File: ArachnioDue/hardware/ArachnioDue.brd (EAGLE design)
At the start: 17.8 x 58.4 mm, 70 parts, among them J5 HEAD17-NOSS, J6 HEAD17-NOSS, Q1 12MHz, U1 SAM3SA-MU, U2 AP2111HA-3.3, U5 ESP8266EX, U6 SPI_FLASH, Y1 26 MHz/10 pF

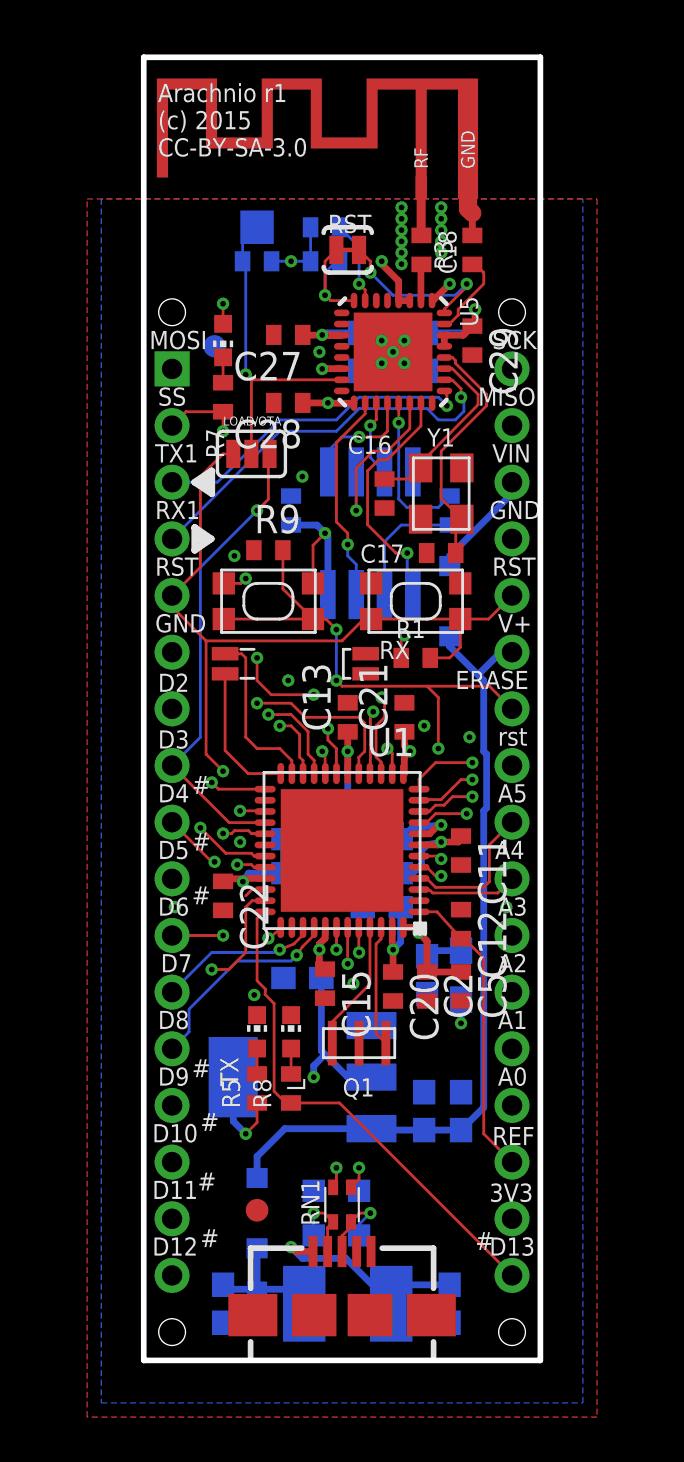
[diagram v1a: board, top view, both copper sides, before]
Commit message: first module version, ready for mfg
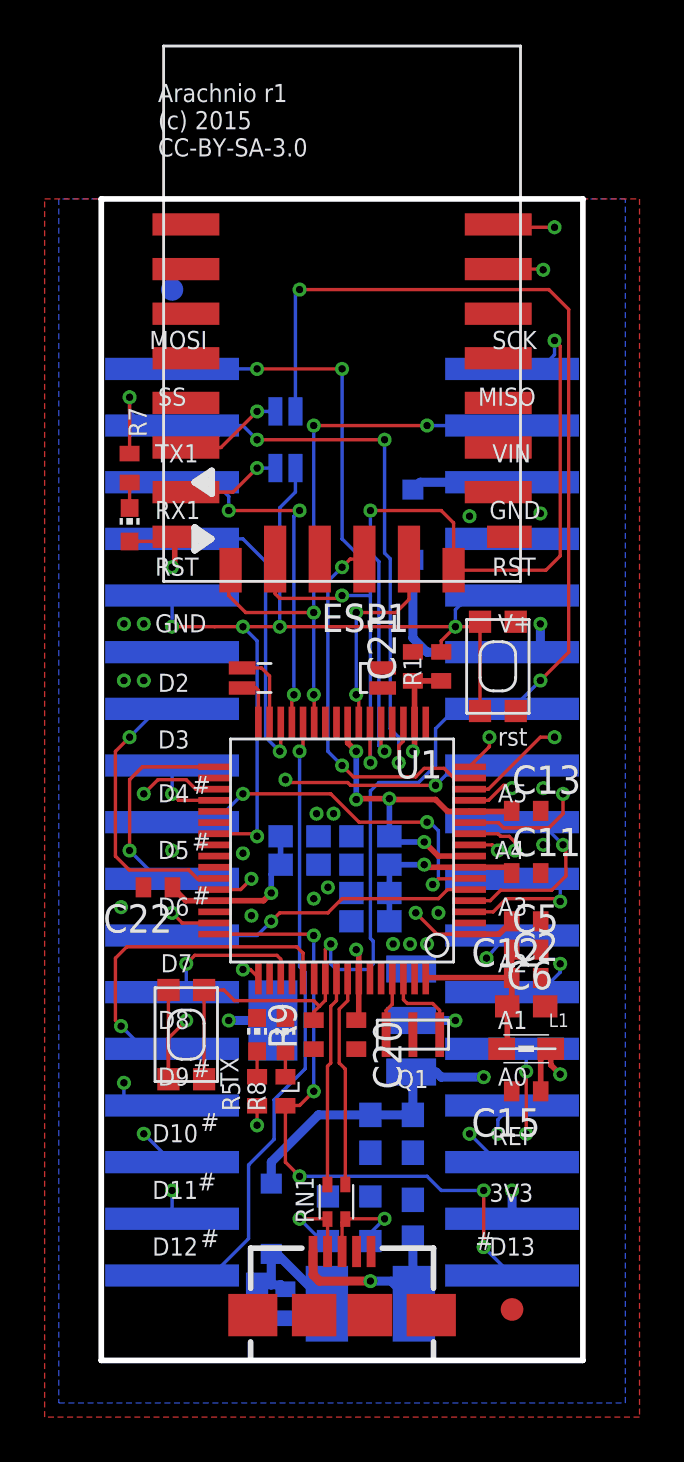
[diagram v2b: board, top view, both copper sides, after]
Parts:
- removed C16, C17: 10 pF, resistor:C0402
- removed C18: 5p6, resistor:C0402
- removed C19, C27, C28, C29: 100n, resistor:C0402
- removed C25, C26: 4u7, resistor:C0603
- removed LOAD/OTA: (no value), SparkFun-Passives:PAD-JUMPER-3-NO_YES_SILK
- removed R10, R11, R14: 10K, resistor:R0402
- removed R13: 200R, resistor:R0402
- removed R3: 12K, resistor:R0402
- removed RST: (no value), SparkFun-Passives:PAD-JUMPER-2-NC_BY_TRACE_YES_SILK
- removed TP3: PTR1TP15SQ, testpad:TP15SQ
- removed U$11: ANTENNA_1RIGHT, ant-planar-1:SWRA117D_RIGHT
- removed U5: ESP8266EX, ESP8266:QFN32
- removed U6: SPI_FLASH, ESP8266:SOIC-8
- removed Y1: 26 MHz/10 pF, SmartPrj:CRYSTAL-3.2-2.5
- added ERASE_JMP, RST_JMP: JUMPER-PAD-2-NOYES_SILK, SparkFun-Passives:PAD-JUMPER-2-NO_YES_SILK
- added ESP1: ESP-12, esp8266-parts:ESP-12
- J5: value HEAD17-NOSS -> (none); device SmartPrj:HEAD17-NOSS -> logos-headers:1X17SMD-UNIVERSAL
- J6: device SmartPrj:HEAD17-NOSS-1 -> logos-headers:1X17SMD-UNIVERSAL
- U1: value SAM3SA-MU -> SAM3SB-AU; device atmel-sam3s:QFN48 -> atmel-sam3s:LQFP64
- moved R9 21.8 mm to (7.62, 14.6), turned to 90 degrees
- moved ERASE 19.8 mm to (1.91, 14.6), turned to 90 degrees
- moved U$12 15.1 mm to (17.1, 48.3)
- moved U$37 12.3 mm to (16.5, 2.29)
- moved C15 10.2 mm to (17.1, 12.1), turned to 180 degrees
- moved RX 9.26 mm to (-0.64, 37.5), turned to 0 degrees
- moved C13 9.03 mm to (17.1, 24.6), turned to 0 degrees
- moved U$1 6.25 mm to (14.6, 41.3)
- moved R7 5.26 mm to (-0.64, 40.0), turned to 270 degrees
- moved RESET 4.70 mm to (15.9, 31.1), turned to 270 degrees
- moved C6 4.66 mm to (17.1, 15.9), flipped to the top, turned to 0 degrees
- moved C2 4.46 mm to (17.1, 17.1), turned to 0 degrees
- moved L1 4.41 mm to (17.1, 14.0), flipped to the top, turned to 180 degrees
- moved C8 4.15 mm to (12.1, 6.35), turned to 90 degrees
- moved C1 3.97 mm to (10.2, 19.7)
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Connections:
- removed net DVDD: U5.24
- removed net N$27: C17.1, U5.28, Y1.1
- removed net N$28: C16.1, U5.27, Y1.3
- removed net N$31: C18.1, U$11.RF
- removed net N$32: R3.1, U5.31
- removed net N$33: RST.1, U5.32
- removed net N$34: R13.2, U5.21
- removed net N$35: R13.1, U6.6
- removed net N$36: U5.20, U6.1
- removed net N$37: U5.18, U6.7
- removed net N$38: U5.19, U6.3
- removed net N$39: U5.23, U6.5
- removed net N$40: U5.22, U6.2
- removed net N$45: C18.2, U5.2
- removed net N$6: LOAD/OTA.2, R10.1, TP3.TP, U5.15
- removed net SWO/ESP_RST: J6.8, R14.2, RST.2, U1.37, U5.8
- removed net VDD: U5.16
- removed net VDD_RTC: U5.5
- new net ESP_CS: ESP1.CS, U1.15
- new net ESP_INT: ESP1.INT, U1.23
- new net ESP_LOAD: ESP1.GPIO0
- new net ESP_RESET: ESP1.REST
- new net ESP_RX: ESP1.TXD, U1.11
- new net ESP_TX: ESP1.RXD, U1.14
- new net N$4: ESP1.GPIO13, RST_JMP.2
- new net N$8: ERASE_JMP.1, ESP1.GPIO12
- new net SWO: J6.8, U1.49
- net 3V3: now also ESP1.VCC, U1.18, U1.45, U1.58; no longer C19.1, C25.1, C26.1, C27.1, C28.1, C29.1, R10.2, R11.1, R14.1, U1.13, U1.33, U1.47, U5.1, U5.11, U5.14, U5.17, U5.29, U5.3, U5.30, U5.4, U6.8
- net A2: now also U1.13; no longer U1.11
- net A3: now also U1.16; no longer U1.12
- net CHIP_EN: now also U1.20; no longer R11.2, U1.15, U5.7
- net D0/RX: now also U1.30; no longer U1.22, U5.26
- net D1/TX: now also U1.29; no longer U1.21, U5.25
- net D10: now also U1.44; no longer U1.32
- net D11: now also U1.47; no longer U1.35
- net D12: now also U1.28; no longer U1.20
- net D13: now also U1.48; no longer U1.36
- net D2/SDA: now also U1.43; no longer U1.31
- net D3/SCL: now also U1.36; no longer LOAD/OTA.3, U1.28
- net D5: now also U1.33; no longer U1.25
- net D9: now also U1.35; no longer U1.27
- net ERASE: now also ERASE_JMP.2, U1.55; no longer U1.42
- net GND: now also ESP1.GND, U1.17, U1.40, U1.46, U1.60; no longer C16.2, C17.2, C19.2, C25.2, C26.2, C27.2, C28.2, C29.2, R3.2, U$11.GND, U1.30, U1.34, U5.13, U5.33, U6.4, Y1.2, Y1.4
- net MISO: now also ESP1.MOSI, U1.27; no longer U1.19
- net MOSI: now also ESP1.MISO, U1.22; no longer U1.17
- net N$1: now also U1.31; no longer U1.23
- net N$5: now also U1.32; no longer U1.24
- net RD+: now also U1.57; no longer U1.44
- net RD-: now also U1.56; no longer U1.43
- net RESET: now also RST_JMP.1, U1.39; no longer LOAD/OTA.1, U1.29
- net RXTXLED/SS: now also U1.19; no longer U1.14
- net SCK: now also ESP1.CLK, U1.21; no longer U1.16
- net SWCLK/D8: now also U1.53; no longer U1.40
- net SWDIO/D7: now also U1.51; no longer U1.39
- net VDDOUT: now also U1.12, U1.24; no longer U1.18, U1.41
- net VDDPLL: now also U1.64; no longer U1.48
- net XTAL1: now also U1.62; no longer U1.46
- net XTAL2: now also U1.61; no longer U1.45
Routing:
- net SWO/ESP_RST: track 52.4 -> 0.00 mm, vias 2 -> 0
- net ESP_RX: track 0.00 -> 34.5 mm, vias 0 -> 2
- net ERASE: track 37.1 -> 69.8 mm, vias 4 -> 3
- net ESP_TX: track 0.00 -> 28.6 mm, vias 0 -> 2
- net CHIP_EN: track 26.5 -> 0.00 mm, vias 2 -> 0
- net SWO: track 0.00 -> 20.8 mm, vias 0 -> 3
- net 3V3: track 58.6 -> 40.1 mm, vias 17 -> 10
- net D0/RX: track 32.9 -> 14.7 mm, vias 2 -> 1
- net D3/SCL: track 21.0 -> 3.31 mm
- net ESP_CS: track 0.00 -> 16.8 mm, vias 0 -> 2
- net D1/TX: track 32.4 -> 16.3 mm, vias 2 -> 3
- net N$6: track 15.0 -> 0.00 mm, vias 1 -> 0
- net SCK: track 21.4 -> 36.1 mm, vias 1 -> 3
- net N$27: track 11.6 -> 0.00 mm
- net VCC: track 35.9 -> 47.5 mm, vias 0 -> 2
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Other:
- board size 17.8 x 58.4 mm -> 21.6 x 52.1 mm
- board text removed: "ERASE"
- board text removed: "RX"
